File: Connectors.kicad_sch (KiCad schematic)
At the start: 1 part, among them J3 Conn_02x17_Odd_Even

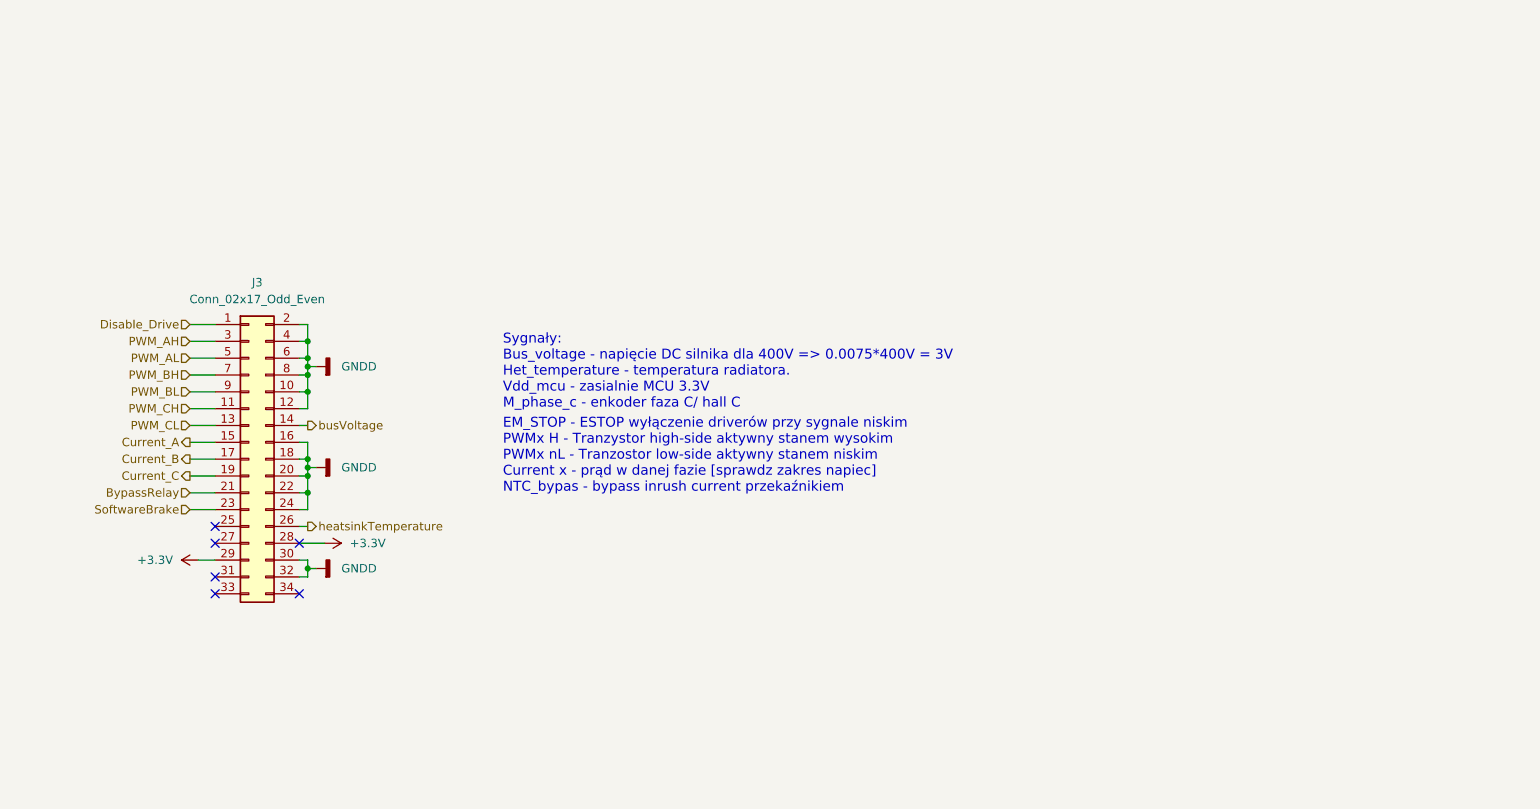
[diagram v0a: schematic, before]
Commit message: 90% schematic first layout
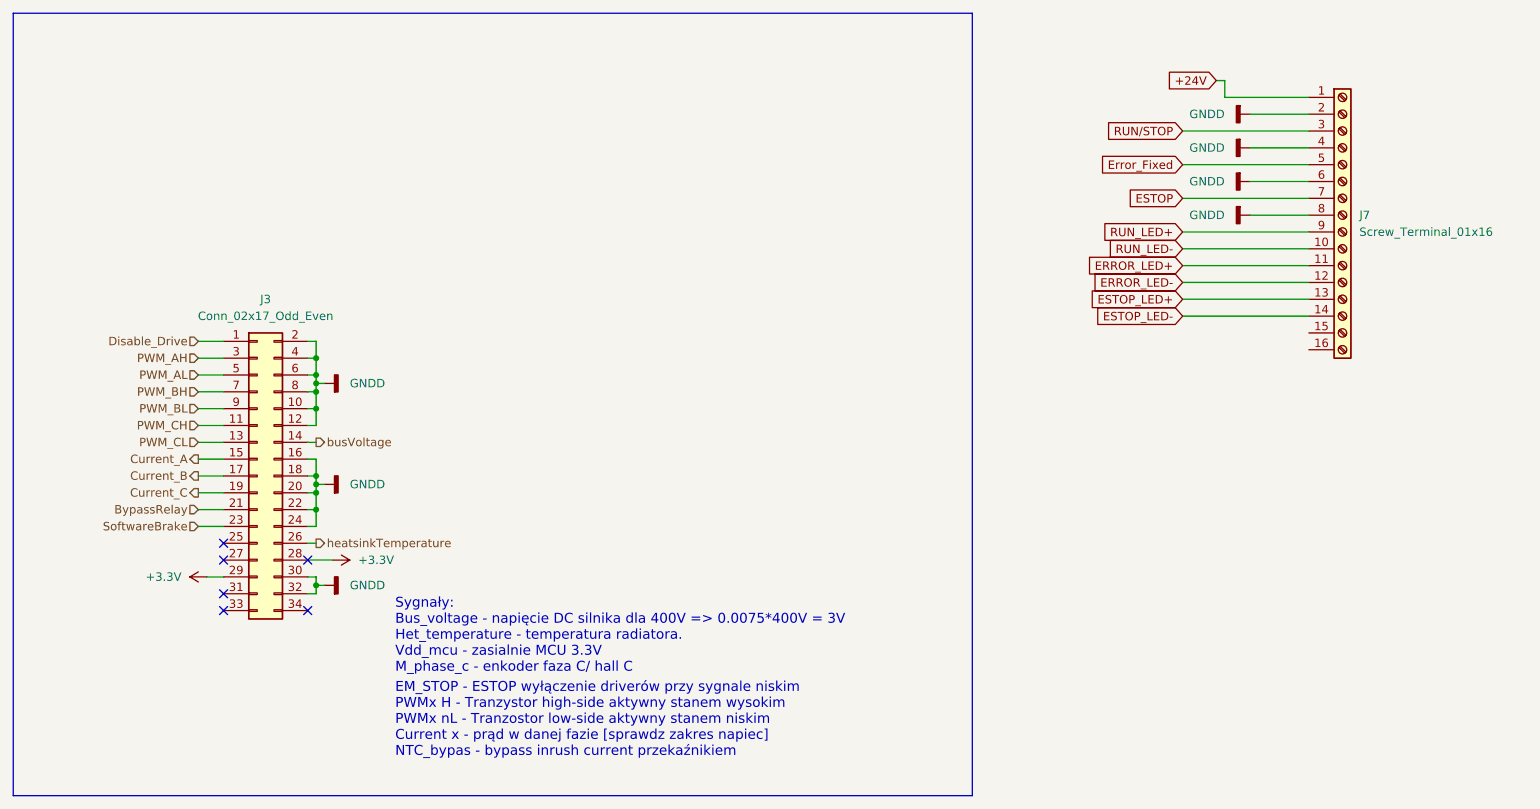
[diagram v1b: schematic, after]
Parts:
- added J7: Screw_Terminal_01x16, TerminalBlock:TerminalBlock_Xinya_XY308-2.54-16P_1x16_P2.54mm_Horizontal, symbol Connector:Screw_Terminal_01x16
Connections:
- net GNDD: now also J7.2 (Pin_2), J7.4 (Pin_4), J7.6 (Pin_6), J7.8 (Pin_8)
- new net +24V: J7.1 (Pin_1)
- new net ERROR_LED+: J7.11 (Pin_11)
- new net ERROR_LED-: J7.12 (Pin_12)
- new net ESTOP: J7.7 (Pin_7)
- new net ESTOP_LED+: J7.13 (Pin_13)
- new net ESTOP_LED-: J7.14 (Pin_14)
- new net Error_Fixed: J7.5 (Pin_5)
- new net RUN_LED+: J7.9 (Pin_9)
- new net RUN_LED-: J7.10 (Pin_10)
- new net RUN/STOP: J7.3 (Pin_3)
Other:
- moved on the sheet: J3
